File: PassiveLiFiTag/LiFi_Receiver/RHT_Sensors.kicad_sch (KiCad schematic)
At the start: 12 parts, among them U4 HDC2080DMBR, U5 HDC2080DMBR

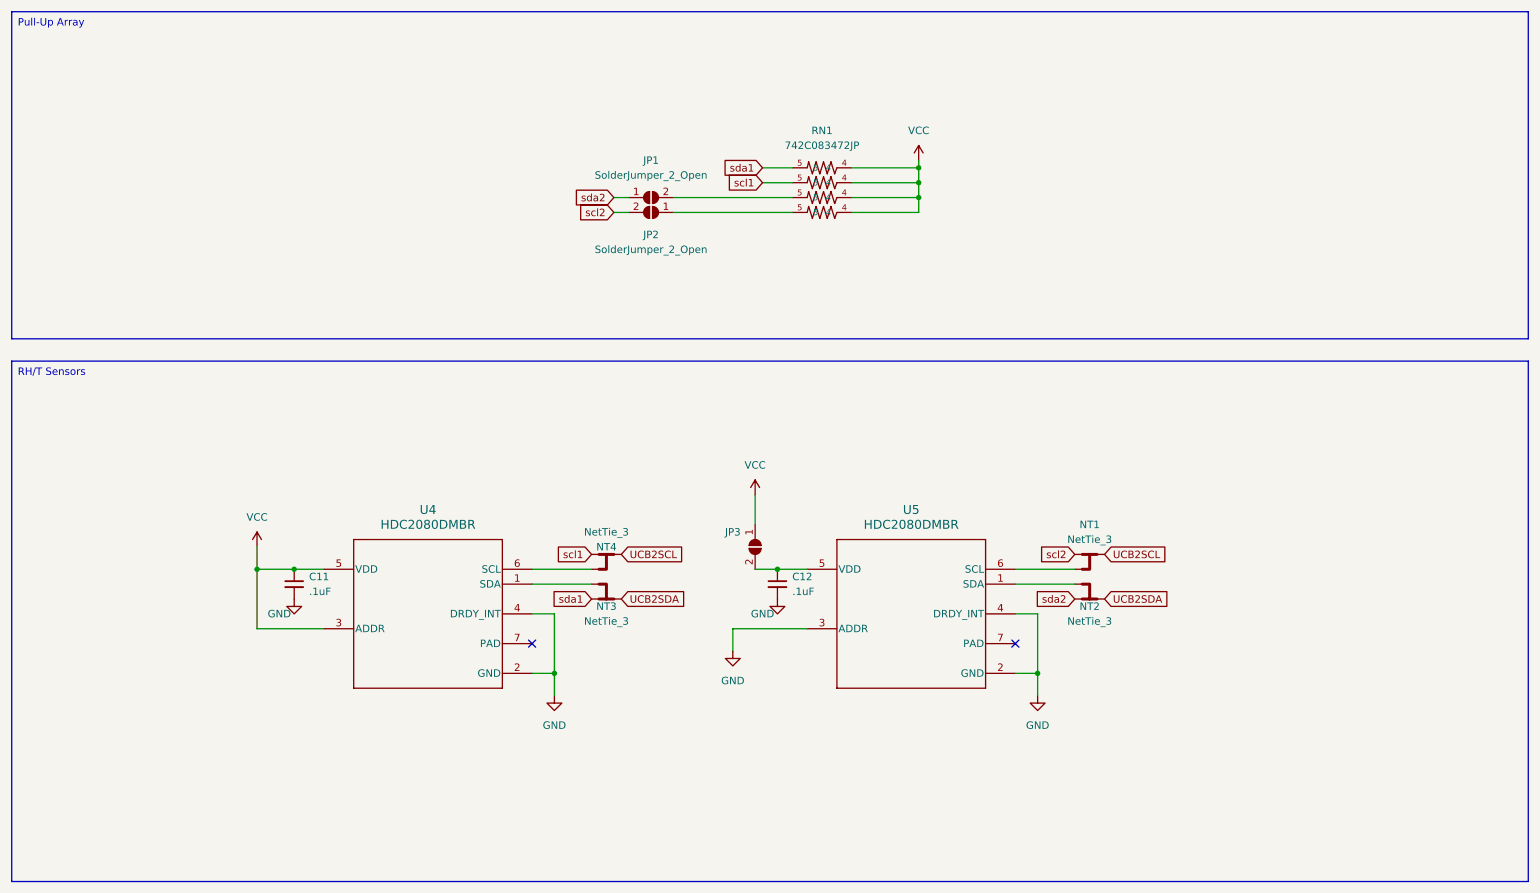
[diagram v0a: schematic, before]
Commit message: Design almost completed
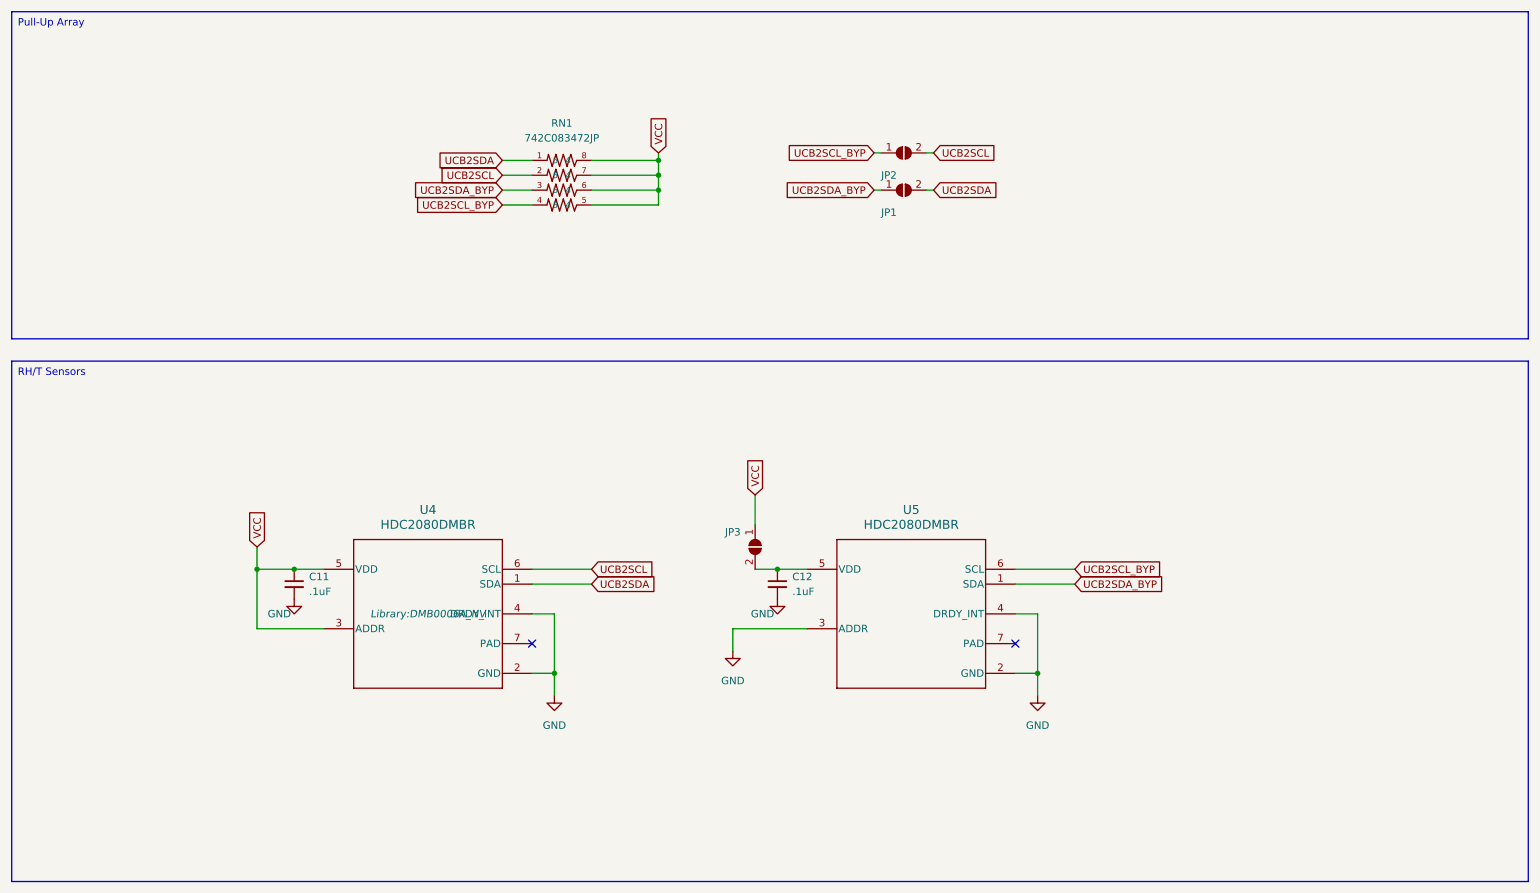
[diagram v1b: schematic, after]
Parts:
- removed NT1, NT2, NT3, NT4: NetTie_3, symbol Device:NetTie_3
- C11, C12: footprint Capacitor_SMD:C_01005_0402Metric -> Capacitor_SMD:C_0603_1608Metric
- RN1: footprint LIFI-FOOTPRINTS:Res_network -> Library:RESCAV80P320X160X70-8N
- U4, U5: footprint LIFI-FOOTPRINTS:HDC2080_1 -> Library:DMB0006A_NV
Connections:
- net scl1 is gone; now on net VCC: RN1.5 (4)
- net scl2 is gone; now on net UCB2SCL: JP2.2 (B)
- net sda1 is gone; now on net VCC: RN1.5 (4)
- net sda2 is gone; now on net UCB2SDA_BYP: JP1.1 (A)
- net UCB2SCL: now also RN1.2 (5), U4.6 (SCL)
- net UCB2SDA: now also JP1.2 (B), RN1.1 (5), U4.1 (SDA)
- net VCC: now also RN1.6 (4), RN1.7 (4), RN1.8 (4); no longer RN1.4
- net UCB2SCL_BYP: now reaches U5.6 (SCL)
- net UCB2SCL_BYP: now also JP2.1 (A), RN1.4 (5)
- net UCB2SDA_BYP: now reaches U5.1 (SDA)
- net UCB2SDA_BYP: now also RN1.3 (5)
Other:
- moved on the sheet: RN1
